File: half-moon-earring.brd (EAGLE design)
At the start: 70 x 70 mm, 10 parts, among them IC1 TTP223, T1 BC817

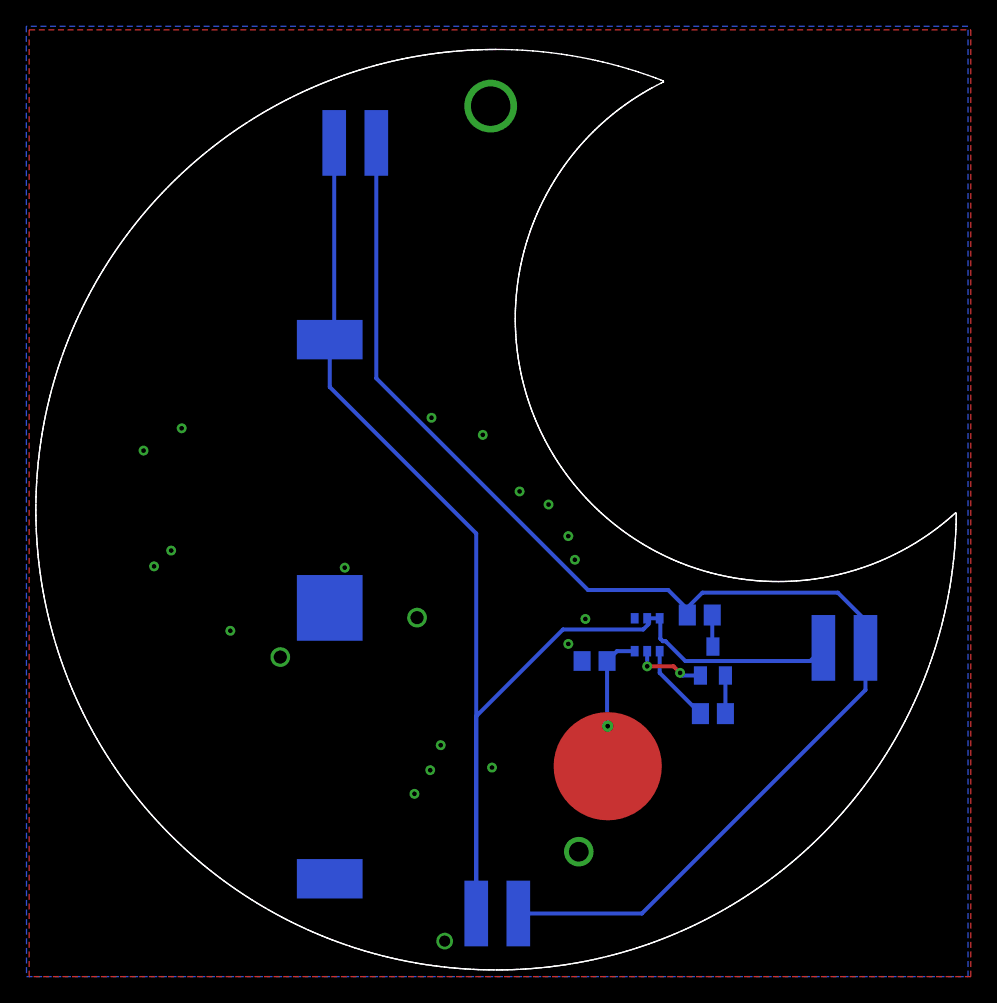
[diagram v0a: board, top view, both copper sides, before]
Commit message: correção de tamanho
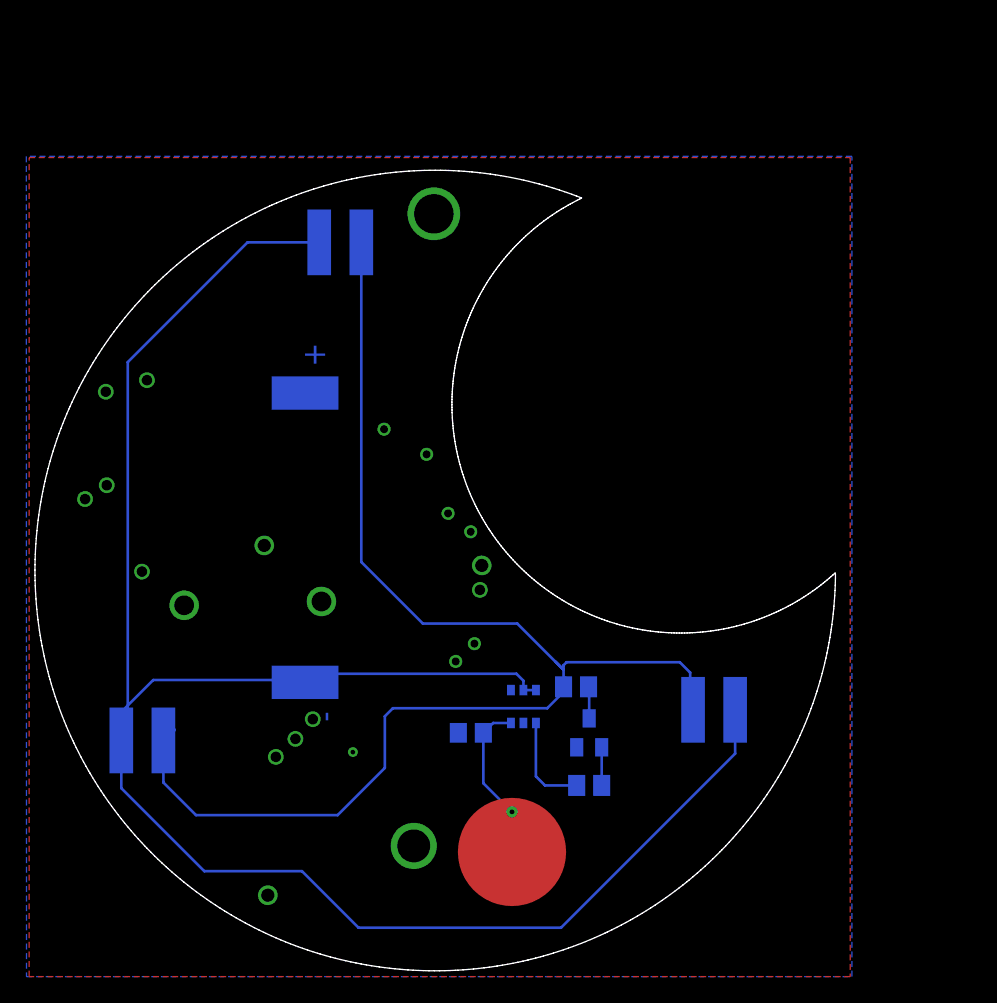
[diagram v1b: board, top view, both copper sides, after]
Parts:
- removed PW1: CR2025 BATERY HOLDER, supply1:CR2025
- added U$1: CR2035, cr2025:CR2035
- moved LED3 30.0 mm to (8.61, 18.0)
- moved LED1 11.0 mm to (52.1, 20.3), turned to 0 degrees
- moved C1 10.9 mm to (33.6, 18.5)
- moved IC1 10.9 mm to (37.6, 20.5)
- moved R1 10.9 mm to (42.6, 14.5)
- moved R2 10.9 mm to (41.6, 22.0)
- moved T1 10.9 mm to (42.6, 18.5)
- moved B2 9.77 mm to (36.7, 9.48)
- moved LED2 7.65 mm to (23.7, 55.8)
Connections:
- net GND: now also U$1.P$2; no longer PW1.P$3
- net VCC: now also U$1.P$1; no longer PW1.P$1
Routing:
- net VCC: track 111.5 -> 147.8 mm
- net GND: track 5.49 -> 0.00 mm, vias 2 -> 0
- net N$11: track 7.38 -> 9.33 mm
- net DRIVER: track 6.03 -> 7.45 mm
- net LEDS: track 104.1 -> 103.3 mm
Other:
- board size 70 x 70 mm -> 60.9 x 60.9 mm
